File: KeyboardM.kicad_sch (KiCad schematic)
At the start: 12 parts, among them U1 ATmega32U4-A

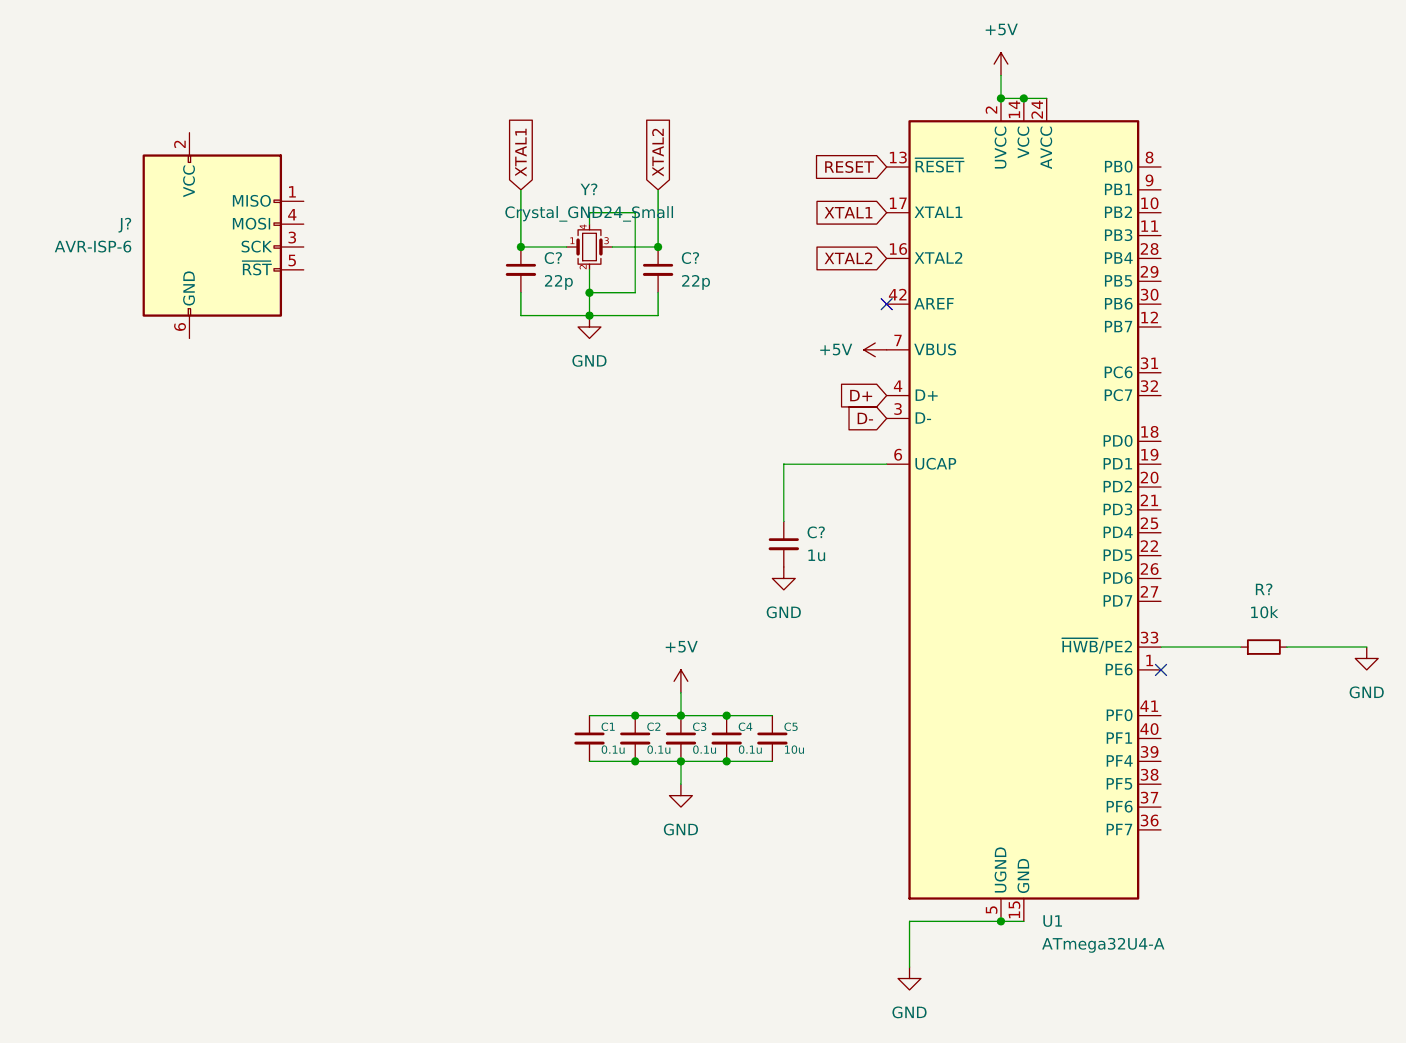
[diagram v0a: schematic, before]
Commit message: ISP Header
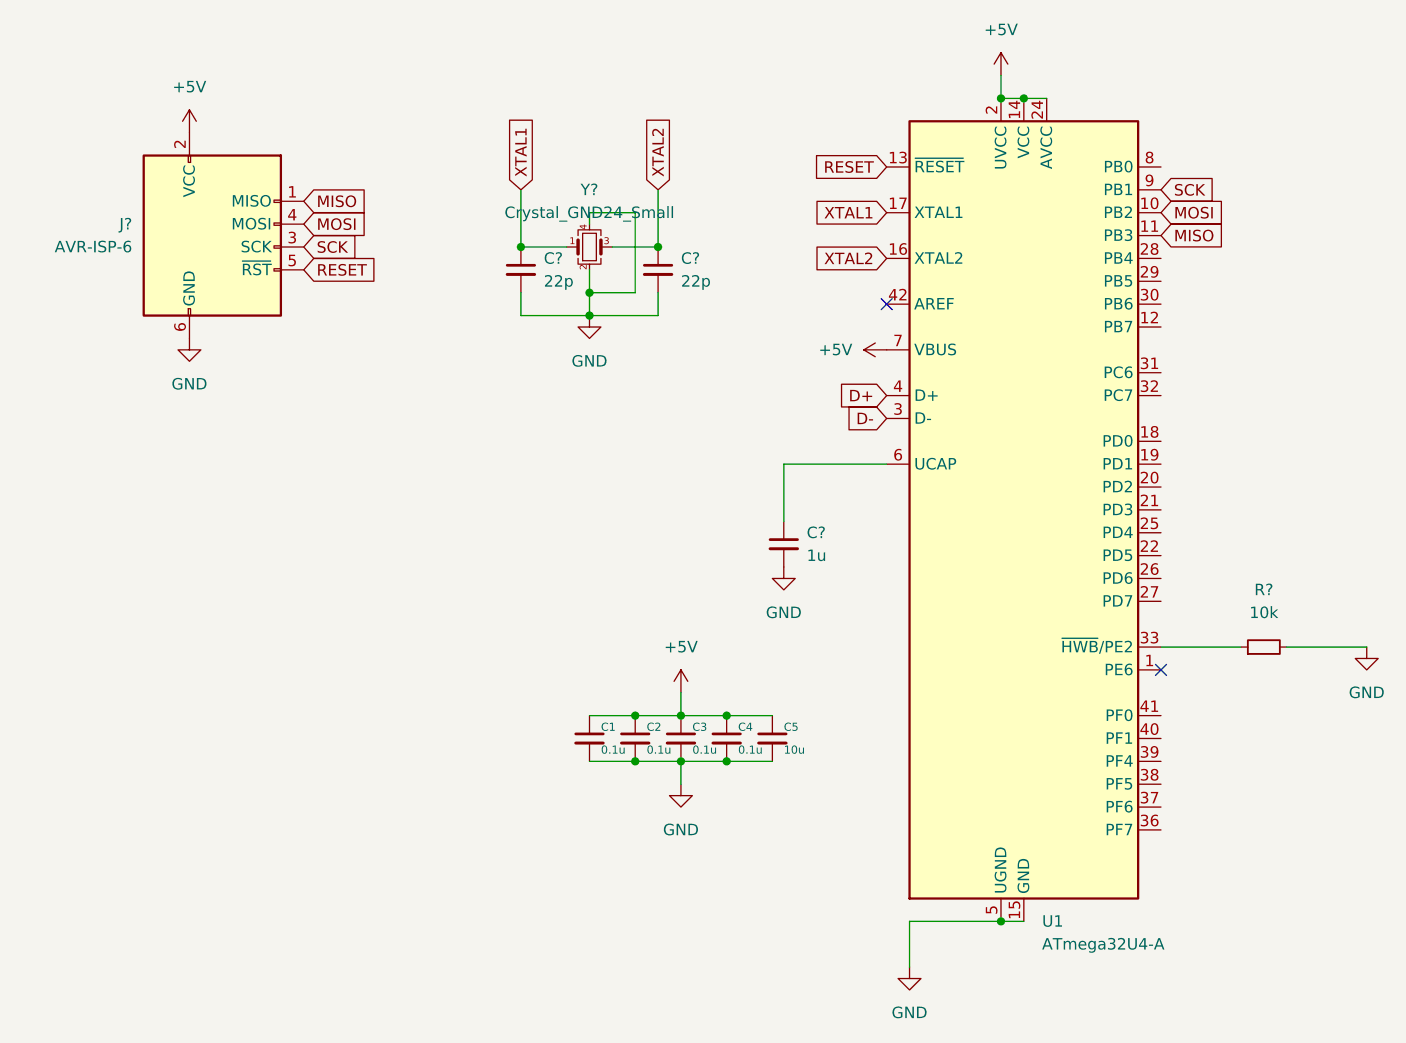
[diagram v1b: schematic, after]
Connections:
- net +5V: now also J?.2 (VCC)
- net GND: now also J?.6 (GND)
- net RESET: now also J?.5 (~{RST})
- net MISO: now reaches J?.1 (MISO)
- net MISO: now also U1.11 (PB3)
- net SCK: now reaches J?.3 (SCK)
- net SCK: now also U1.9 (PB1)
- net MOSI: now reaches J?.4 (MOSI)
- net MOSI: now also U1.10 (PB2)
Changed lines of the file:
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@@
     (stroke (width 0) (type default) (color 0 0 0 0))
+  )
+  (global_label "RESET" (shape input) (at 63.5 78.74 0) (fields_autoplaced)
+    (effects (font (size 1.27 1.27)) (justify left))
+    (property "Intersheet References" "${INTERSHEET_REFS}" (id 0) (at 71.6583 78.6606 0)
+      (effects (font (size 1.27 1.27)) (justify left) hide)
+    )
   )
   (global_label "XTAL2" (shape input) (at 102.87 69.85 90) (fields_autoplaced)
@@
     )
   )
+  (global_label "MISO" (shape input) (at 63.5 71.12 0) (fields_autoplaced)
+    (effects (font (size 1.27 1.27)) (justify left))
+    (property "Intersheet References" "${INTERSHEET_REFS}" (id 0) (at 70.5093 71.0406 0)
+      (effects (font (size 1.27 1.27)) (justify left) hide)
+    )
+  )
   (global_label "XTAL1" (shape input) (at 128.27 72.39 180) (fields_autoplaced)
     (effects (font (size 1.27 1.27)) (justify right))
@@
     )
   )
+  (global_label "SCK" (shape input) (at 63.5 76.2 0) (fields_autoplaced)
+    (effects (font (size 1.27 1.27)) (justify left))
+    (property "Intersheet References" "${INTERSHEET_REFS}" (id 0) (at 69.6626 76.1206 0)
+      (effects (font (size 1.27 1.27)) (justify left) hide)
+    )
+  )
+  (global_label "MOSI" (shape input) (at 63.5 73.66 0) (fields_autoplaced)
+    (effects (font (size 1.27 1.27)) (justify left))
+    (property "Intersheet References" "${INTERSHEET_REFS}" (id 0) (at 70.5093 73.5806 0)
+      (effects (font (size 1.27 1.27)) (justify left) hide)
+    )
+  )
   (global_label "XTAL2" (shape input) (at 128.27 77.47 180) (fields_autoplaced)
     (effects (font (size 1.27 1.27)) (justify right))
@@
     )
   )
+  (global_label "MISO" (shape input) (at 158.75 74.93 0) (fields_autoplaced)
+    (effects (font (size 1.27 1.27)) (justify left))
+    (property "Intersheet References" "${INTERSHEET_REFS}" (id 0) (at 165.7593 74.8506 0)
+      (effects (font (size 1.27 1.27)) (justify left) hide)
+    )
+  )
+  (global_label "SCK" (shape input) (at 158.75 69.85 0) (fields_autoplaced)
+    (effects (font (size 1.27 1.27)) (justify left))
+    (property "Intersheet References" "${INTERSHEET_REFS}" (id 0) (at 164.9126 69.7706 0)
+      (effects (font (size 1.27 1.27)) (justify left) hide)
+    )
+  )
+  (global_label "MOSI" (shape input) (at 158.75 72.39 0) (fields_autoplaced)
+    (effects (font (size 1.27 1.27)) (justify left))
+    (property "Intersheet References" "${INTERSHEET_REFS}" (id 0) (at 165.7593 72.3106 0)
+      (effects (font (size 1.27 1.27)) (justify left) hide)
+    )
+  )
   (global_label "XTAL1" (shape input) (at 87.63 69.85 90) (fields_autoplaced)
     (effects (font (size 1.27 1.27)) (justify left))
@@
     (pin "5")
     (pin "6")
+  )
+  (symbol (lib_id "power:GND") (at 50.8 86.36 0) (unit 1)
+    (in_bom yes) (on_board yes) (fields_autoplaced)
+    (property "Reference" "#PWR?" (id 0) (at 50.8 92.71 0)
+      (effects (font (size 1.27 1.27)) hide)
+    )
+    (property "Value" "GND" (id 1) (at 50.8 91.44 0))
+    (property "Footprint" "" (id 2) (at 50.8 86.36 0)
+      (effects (font (size 1.27 1.27)) hide)
+    )
+    (property "Datasheet" "" (id 3) (at 50.8 86.36 0)
+      (effects (font (size 1.27 1.27)) hide)
+    )
+    (pin "1")
   )
   (symbol (lib_id "Device:C_Small") (at 100.33 130.81 0) (unit 1)
@@
     (pin "9")
   )
+  (symbol (lib_id "power:+5V") (at 50.8 63.5 0) (unit 1)
+    (in_bom yes) (on_board yes) (fields_autoplaced)
+    (property "Reference" "#PWR?" (id 0) (at 50.8 67.31 0)
+      (effects (font (size 1.27 1.27)) hide)
+    )
+    (property "Value" "+5V" (id 1) (at 50.8 58.42 0))
+    (property "Footprint" "" (id 2) (at 50.8 63.5 0)
+      (effects (font (size 1.27 1.27)) hide)
+    )
+    (property "Datasheet" "" (id 3) (at 50.8 63.5 0)
+      (effects (font (size 1.27 1.27)) hide)
+    )
+    (pin "1")
+  )
   (symbol (lib_id "Device:C_Small") (at 102.87 78.74 0) (unit 1)
     (in_bom yes) (on_board yes) (fields_autoplaced)
@@
       (reference "#PWR?") (unit 1) (value "GND") (footprint "")
     )
+    (path "/3bd5d607-5d90-461d-9e03-623ce54f8a63"
+      (reference "#PWR?") (unit 1) (value "GND") (footprint "")
+    )
     (path "/4dbb1b14-93b7-481b-9fc7-7ec555f93957"
       (reference "#PWR?") (unit 1) (value "+5V") (footprint "")
@@
       (reference "#PWR?") (unit 1) (value "GND") (footprint "")
     )
+    (path "/bde56c9e-c398-4c7d-a88d-532a00b6e85f"
+      (reference "#PWR?") (unit 1) (value "+5V") (footprint "")
+    )
     (path "/29a715ce-be66-4c11-bd1a-2950b0c010d7"
